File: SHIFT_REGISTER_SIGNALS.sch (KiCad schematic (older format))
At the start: 27 parts, among them Q144 SSM3K35AMFV, Q145 SSM3K35AMFV

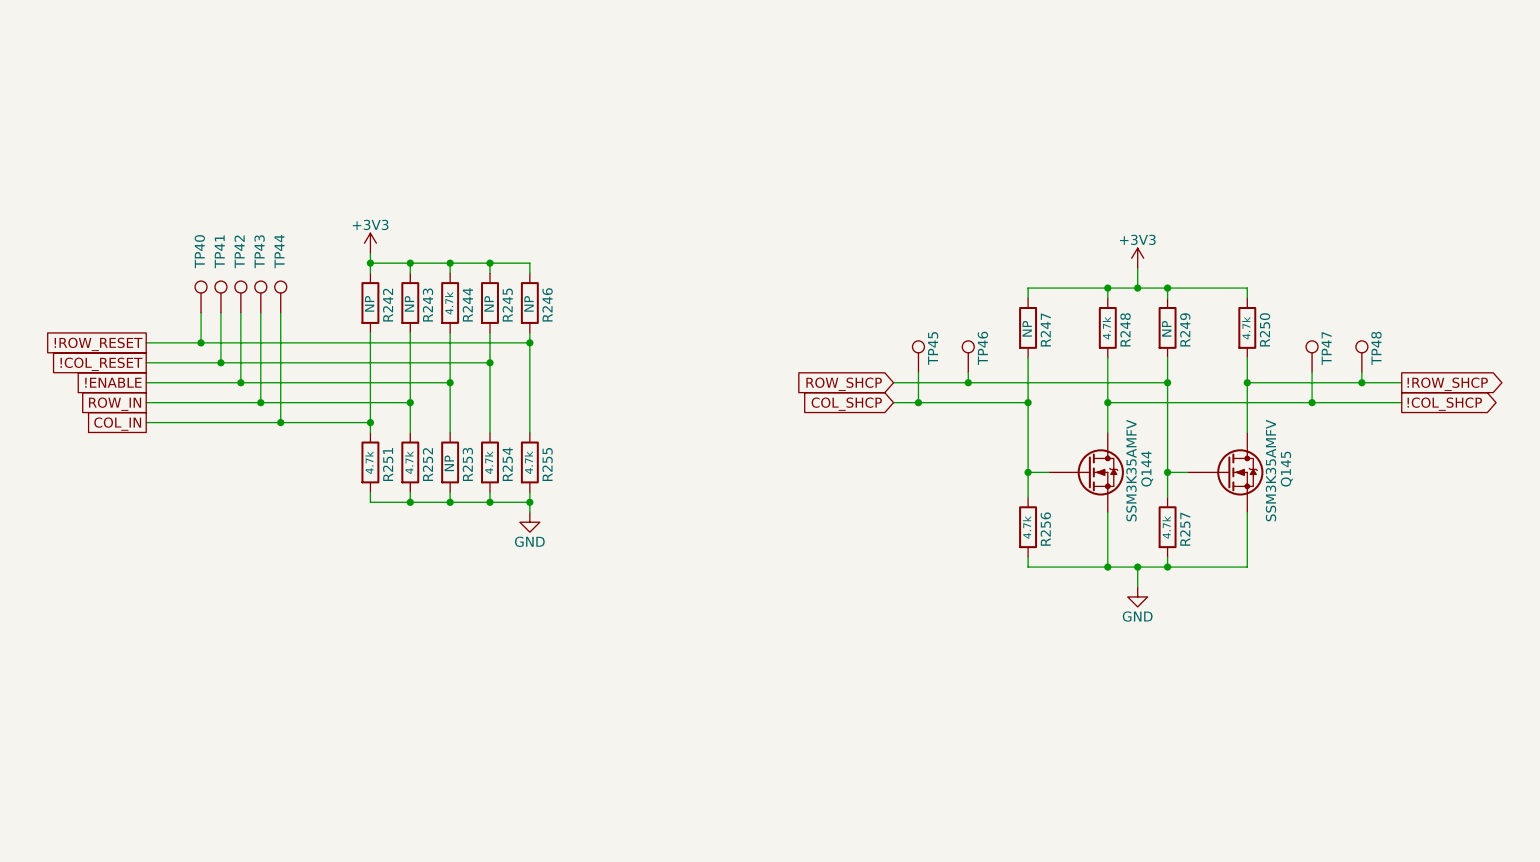
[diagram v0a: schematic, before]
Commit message: automated commit
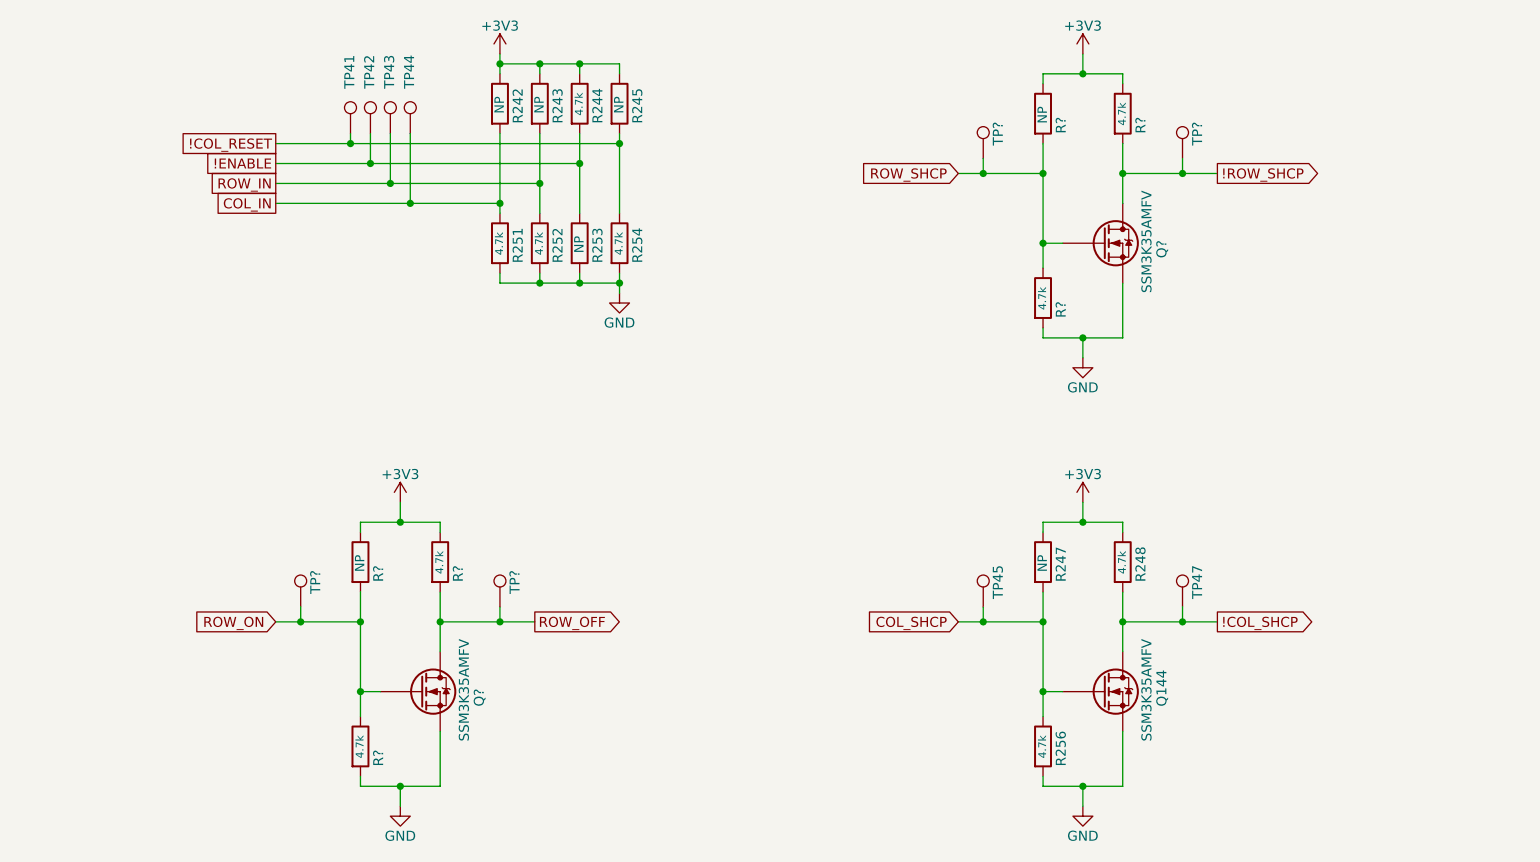
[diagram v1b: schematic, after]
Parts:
- removed Q145: SSM3K35AMFV, symbol custom:SSM3K35AMFV
- removed R246, R249: NP_R_0603, Resistor_SMD:R_0603_1608Metric, symbol custom:NP_R_0603
- removed R250, R255, R257: CRG0603F4K7, Resistor_SMD:R_0603_1608Metric, symbol custom:CRG0603F4K7
- removed TP40, TP46, TP48: TestPoint, symbol Connector:TestPoint
- added Q? (x2): SSM3K35AMFV, symbol custom:SSM3K35AMFV
- added R? (x2): NP_R_0603, Resistor_SMD:R_0603_1608Metric, symbol custom:NP_R_0603
- added R? (x4): CRG0603F4K7, Resistor_SMD:R_0603_1608Metric, symbol custom:CRG0603F4K7
- added TP? (x4): TestPoint, symbol Connector:TestPoint
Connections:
- net !ROW_SHCP: now also Q?.3 (D), R?.2, TP?.1
- net +3V3: now also R?.1, R?.1, R?.1, R?.1
- net GND: now also Q?.2 (S), Q?.2 (S), R?.2, R?.2
- net ROW_SHCP: now also Q?.1 (G), R?.1, R?.2, TP?.1
- new net ROW_OFF: Q?.3 (D), R?.2, TP?.1
- new net ROW_ON: Q?.1 (G), R?.1, R?.2, TP?.1
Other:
- moved on the sheet: Q144, R242, R243, R244, R245, R247, R248, R251, R252, R253, R254, R256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
